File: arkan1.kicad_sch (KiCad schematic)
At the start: 22 parts, among them Q1 NMOS (CHG), Q2 NMOS (DSG), Q3 PMOS, SW1 SW_Push, U1 BQ297xy, U2 SX1276, U3 RXM-GPS-FM, U5 TP4056-42-ESOP8

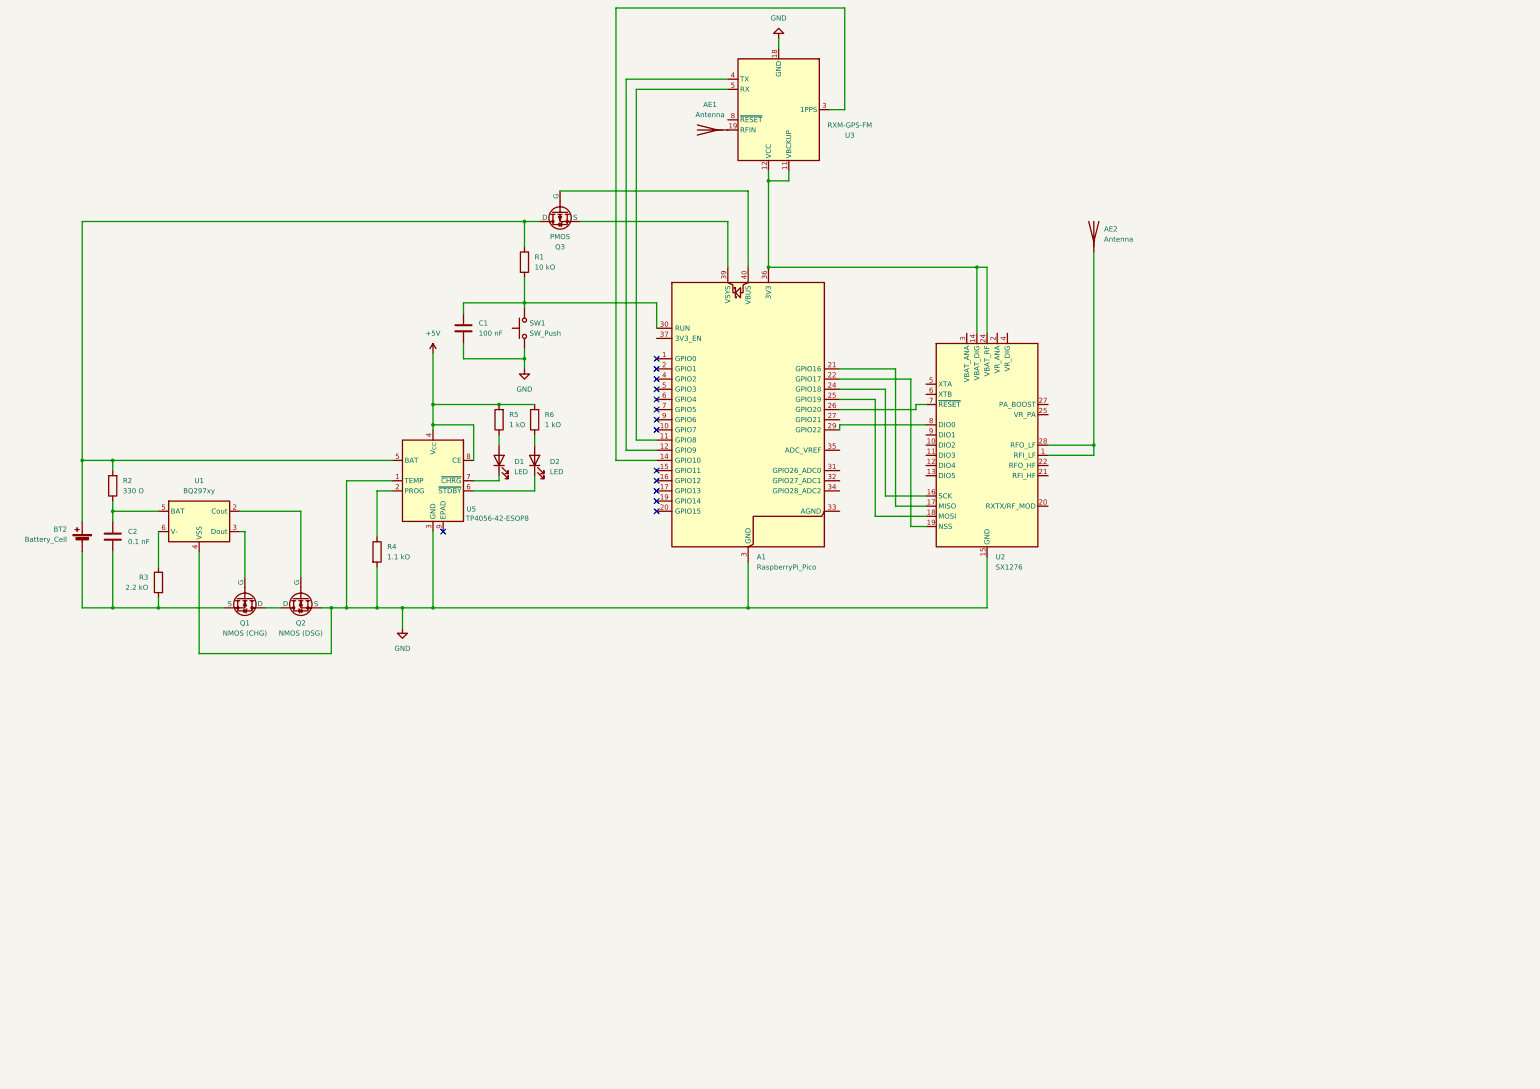
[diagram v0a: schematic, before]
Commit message: Add files via upload
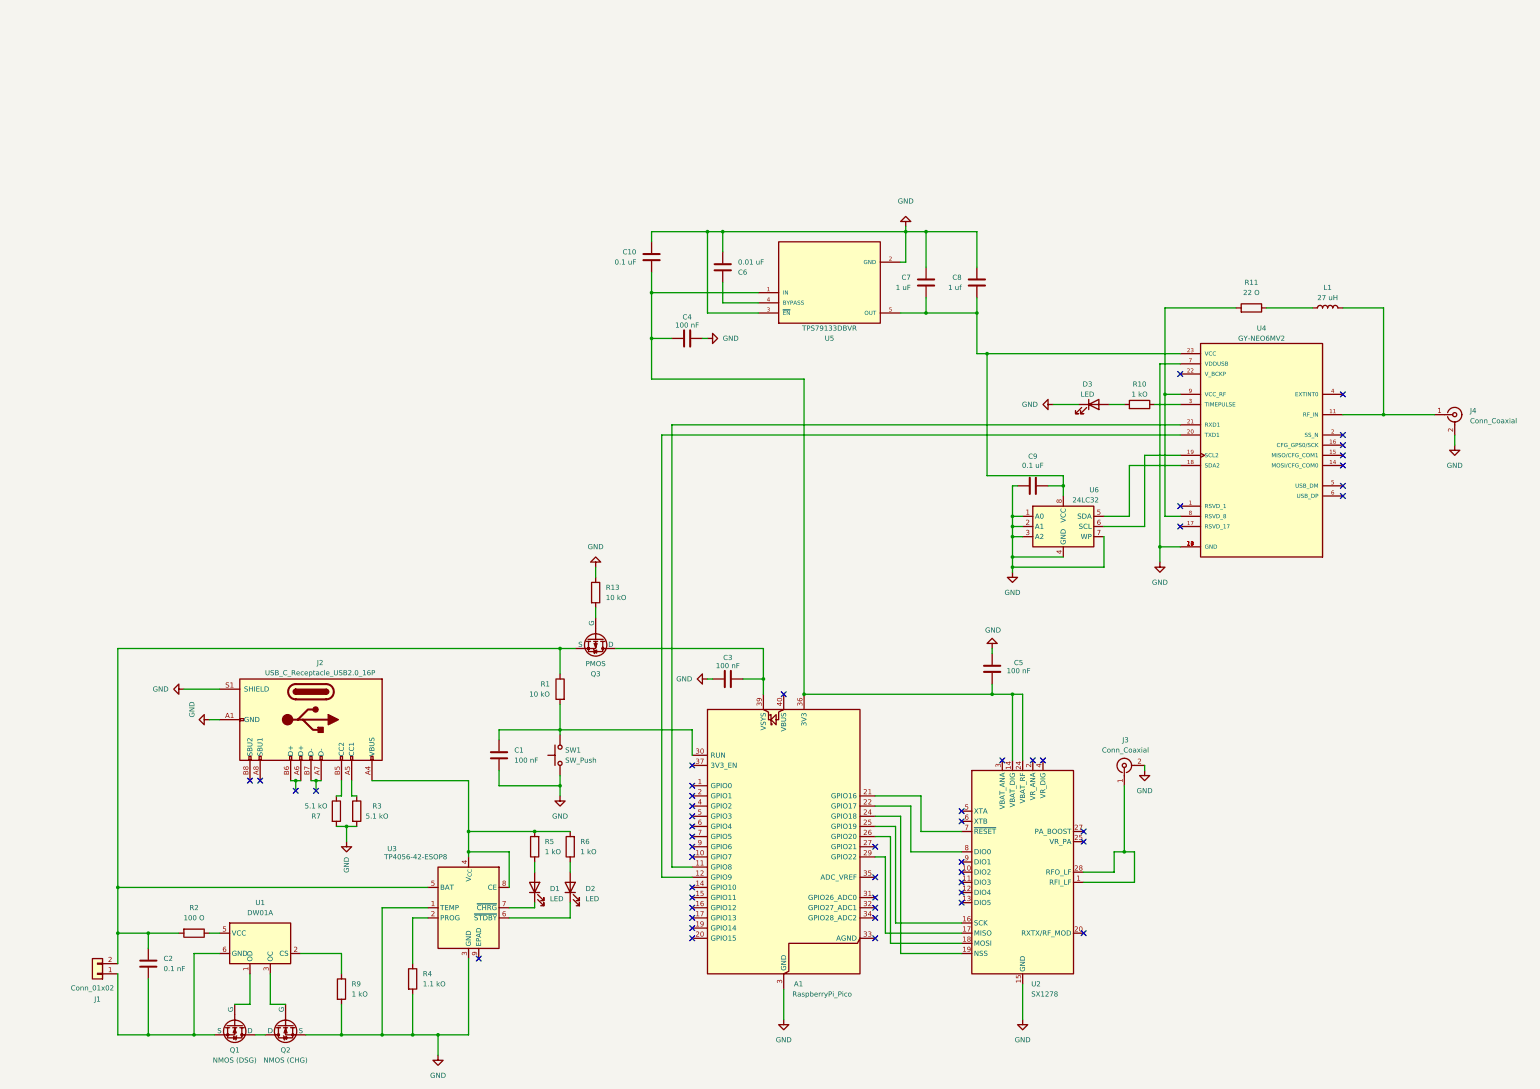
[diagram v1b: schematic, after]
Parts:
- removed AE1, AE2: Antenna, symbol Device:Antenna
- removed BT2: Battery_Cell, symbol Device:Battery_Cell
- removed U1: BQ297xy, Package_SON:WSON-6_1.5x1.5mm_P0.5mm, symbol Battery_Management:BQ297xy
- removed U2: SX1276, Package_DFN_QFN:QFN-28-1EP_6x6mm_P0.65mm_EP4.8x4.8mm, symbol RF:SX1276
- removed U3: RXM-GPS-FM, RF_GPS:Linx_RXM-GPS, symbol RF_GPS:RXM-GPS-FM
- removed U5: TP4056-42-ESOP8, Package_SO:SOIC-8-1EP_3.9x4.9mm_P1.27mm_EP2.41x3.3mm_ThermalVias, symbol Battery_Management:TP4056-42-ESOP8
- added C10, C9: 0.1 uF, Capacitor_SMD:C_0603_1608Metric, symbol Device:C
- added C3: 100 nF, Capacitor_SMD:C_0603_1608Metric, symbol Device:C
- added C4, C5: 100 nF, Capacitor_Tantalum_SMD:CP_EIA-7343-31_Kemet-D, symbol Device:C
- added C6: 0.01 uF, Capacitor_SMD:C_0603_1608Metric, symbol Device:C
- added C7: 1 uF, Capacitor_SMD:C_0603_1608Metric, symbol Device:C
- added C8: 1 uf, Capacitor_SMD:C_0603_1608Metric, symbol Device:C
- added D3: LED, LED_SMD:LED_0201_0603Metric, symbol Device:LED
- added J1: Conn_01x02, Connector_AMASS:AMASS_XT30U-M_1x02_P5.0mm_Vertical, symbol Connector_Generic:Conn_01x02
- added J2: USB_C_Receptacle_USB2.0_16P, Connector_USB:USB_C_Receptacle_GCT_USB4105-xx-A_16P_TopMnt_Horizontal, symbol Connector:USB_C_Receptacle_USB2.0_16P
- added J3, J4: Conn_Coaxial, Connector_Coaxial:SMA_Molex_73251-1153_EdgeMount_Horizontal, symbol Connector:Conn_Coaxial
- added L1: 27 uH, Inductor_SMD:L_1210_3225Metric, symbol Device:L
- added R10, R9: 1 kO, Resistor_SMD:R_0201_0603Metric, symbol Device:R
- added R11: 22 O, Resistor_SMD:R_0201_0603Metric, symbol Device:R
- added R13: 10 kO, Resistor_SMD:R_0201_0603Metric, symbol Device:R
- added R7: 5.1 kO, Resistor_SMD:R_0201_0603Metric, symbol Device:R
- added U1: DW01A, Package_TO_SOT_SMD:SOT-23-6, symbol Battery_Management:DW01A
- added U2: SX1278, Package_DFN_QFN:QFN-28-1EP_6x6mm_P0.65mm_EP4.8x4.8mm, symbol RF:SX1278
- added U3: TP4056-42-ESOP8, Package_SO:SOIC-8-1EP_3.9x4.9mm_P1.27mm_EP2.41x3.3mm_ThermalVias, symbol Battery_Management:TP4056-42-ESOP8
- added U4: GY-NEO6MV2, GY-NEO6MV2 (1):XCVR_GY-NEO6MV2, symbol GY-NEO6MV2:GY-NEO6MV2
- added U5: TPS79133DBVR, TPS79133DBVR:SOT95P280X145-5N, symbol TPS79133DBVR:TPS79133DBVR
- added U6: 24LC32, Package_SO:SOIC-8_3.9x4.9mm_P1.27mm, symbol Memory_EEPROM:24LC32
- A1: footprint Module:RaspberryPi_Pico_Common_Unspecified -> Module:RaspberryPi_Pico_Common_SMD
- C1, C2: footprint (none) -> Capacitor_SMD:C_0603_1608Metric
- D1, D2: footprint (none) -> LED_SMD:LED_0201_0603Metric
- Q1: value NMOS (CHG) -> NMOS (DSG); footprint (none) -> Package_TO_SOT_SMD:SOT-23
- Q2: value NMOS (DSG) -> NMOS (CHG); footprint (none) -> Package_TO_SOT_SMD:SOT-23
- Q3: footprint (none) -> Package_TO_SOT_SMD:SOT-23
- R1, R4, R5, R6: footprint (none) -> Resistor_SMD:R_0201_0603Metric
- R2: value 330 O -> 100 O; footprint (none) -> Resistor_SMD:R_0201_0603Metric
- R3: value 2.2 kO -> 5.1 kO; footprint (none) -> Resistor_SMD:R_0201_0603Metric
- SW1: footprint (none) -> Button_Switch_SMD:SW_SPST_PTS645Sx43SMTR92
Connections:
- net GND: now also R3.2, C10.2, C3.1, C4.1, C5.1, C6.2, C7.2, C8.2, C9.1, D3.1 (K), J2.A1 (GND), J2.A12 (GND), J2.B1 (GND), J2.B12 (GND), J2.S1 (SHIELD), J3.2 (Ext), J4.2 (Ext), R13.1, R7.2, R9.2, U2.15 (GND), U2.21 (GND), U2.22 (GND), U2.23 (GND), U2.26 (GND), U2.29 (GND), U3.1 (TEMP), U3.3 (GND), U4.10 (GND), U4.12 (GND), U4.13 (GND), U4.24 (GND), U4.7 (VDDUSB), U5.2 (GND), U5.3 (~{EN}), U6.1 (A0), U6.2 (A1), U6.3 (A2), U6.4 (GND), U6.7 (WP); no longer A1.13 (GND), A1.18 (GND), A1.23 (GND), A1.28 (GND), A1.3 (GND), A1.38 (GND), A1.8 (GND)
- net at A1.11 (GPIO8): now also U4.21 (RXD1)
- net at A1.12 (GPIO9): now also U4.20 (TXD1)
- net at A1.21 (GPIO16): now also U2.7 (~{RESET})
- net at A1.22 (GPIO17): now also U2.8 (DIO0)
- net at A1.24 (GPIO18): now also U2.19 (NSS)
- net at A1.25 (GPIO19): now also U2.16 (SCK)
- net at A1.26 (GPIO20): now also U2.18 (MOSI)
- net at A1.29 (GPIO22): now also U2.17 (MISO)
- net at A1.36 (3V3): now also C10.1, C4.2, C5.2, U2.14 (VBAT_DIG), U2.24 (VBAT_RF), U5.1 (IN)
- net at Q3.3 (S): now also C2.1, R1.1, R2.2, J1.2 (Pin_2), U3.5 (BAT); no longer A1.39 (VSYS)
- net at A1.40 (VBUS): no longer Q3.2 (G)
- net at Q2.2 (G): now also U1.3 (OC)
- net at Q1.2 (G): now also U1.1 (OD)
- net at R2.1: now also U1.5 (VCC); no longer C2.1
- net at R3.1: now also J2.A5 (CC1)
- net at C2.2, Q1.3 (S): now also J1.1 (Pin_1), U1.6 (GND); no longer R3.2
- net at R4.1: now also U3.2 (PROG)
- net at D2.1 (K): now also U3.6 (~{STDBY})
- net at D1.1 (K): now also U3.7 (~{CHRG})
- net +5V: no longer names the net of R5.2, R6.2
- net +5V: now also J2.A4 (VBUS), J2.A9 (VBUS), J2.B4 (VBUS), J2.B9 (VBUS), U3.4 (V_{CC}), U3.8 (CE)
- new net: A1.13 (GND), A1.18 (GND), A1.23 (GND), A1.28 (GND), A1.3 (GND), A1.38 (GND), A1.8 (GND)
- new net: A1.39 (VSYS), C3.2, Q3.1 (D)
- new net: J2.A6 (D+), J2.B6 (D+)
- new net: J2.A7 (D-), J2.B7 (D-)
- new net: J2.B5 (CC2), R7.1
- new net: Q3.2 (G), R13.2
- new net: J3.1 (In), U2.1 (RFI_LF), U2.28 (RFO_LF)
- new net: R9.1, U1.2 (CS)
- new net: R10.1, U4.3 (TIMEPULSE)
- new net: D3.2 (A), R10.2
- new net: C7.1, C8.1, C9.2, U4.23 (VCC), U5.5 (OUT), U6.8 (VCC)
- new net: J4.1 (In), L1.2, U4.11 (RF_IN)
- new net: U4.18 (SDA2), U6.5 (SDA)
- new net: U4.19 (SCL2), U6.6 (SCL)
- new net: R11.2, U4.8 (RSVD_8), U4.9 (VCC_RF)
- new net: C6.1, U5.4 (BYPASS)
- new net: L1.1, R11.1
- no-connect marks 14 -> 50
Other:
- moved on the sheet: A1, C1, C2, D1, D2, Q1, Q2, Q3, R1, R2, R4, R5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
